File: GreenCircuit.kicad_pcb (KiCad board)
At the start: 2 copper layers, 114.9 x 97.8 mm, 71 parts, among them J1 AVR ISP 6, J2 USB_A-Connector, SW1 SW_Push, SW10 SW_Push, SW11 SW_Push, SW12 SW_Push, SW13 SW_Push, SW14 SW_Push, SW15 SW_Push, SW16 SW_Push, SW17 SW_Push, SW18 SW_Push, SW19 SW_Push, SW2 SW_Push, SW20 SW_Push, SW21 PG1350, SW22 PG1350, SW23 PG1350, SW3 SW_Push, SW4 SW_Push, SW5 SW_Push, SW6 SW_Push, SW7 SW_Push, SW8 SW_Push, SW9 SW_Push, U1 ATmega328P-PU, Y1 16MHz

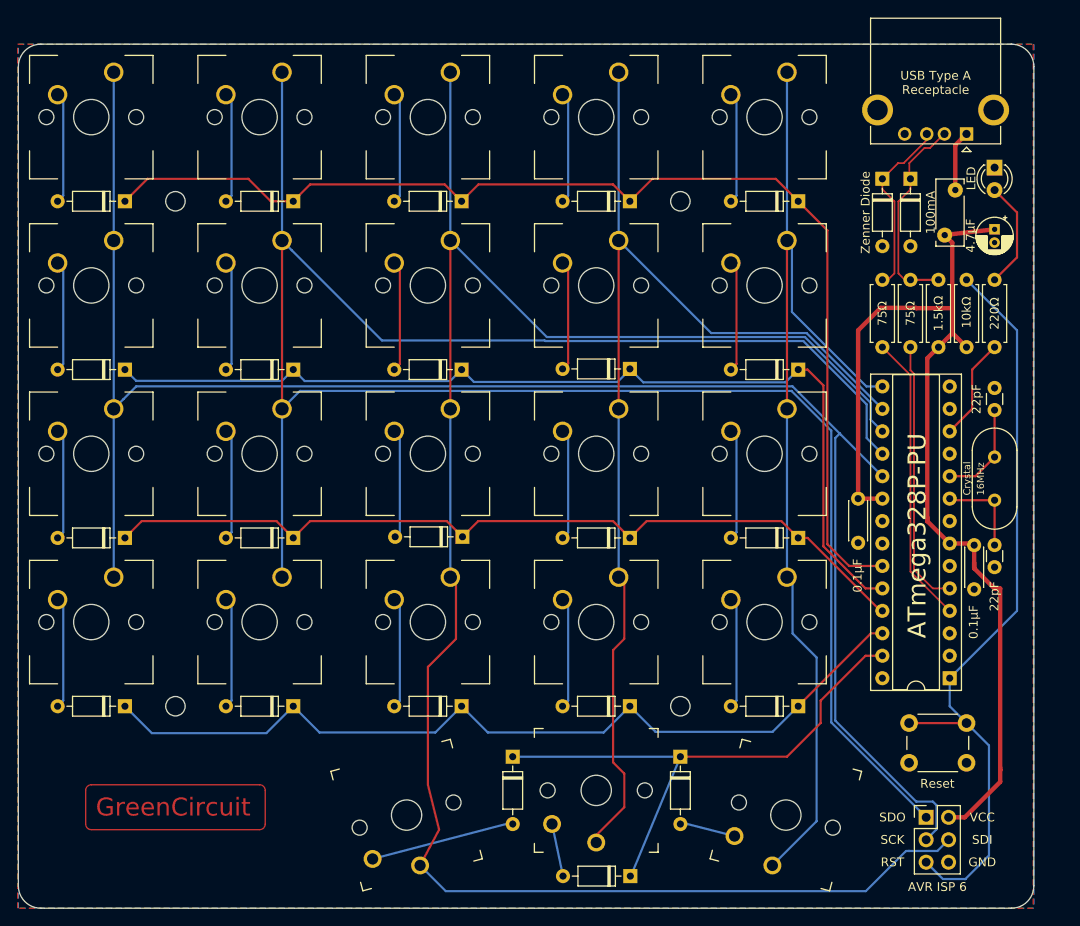
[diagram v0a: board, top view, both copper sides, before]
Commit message: v0.5
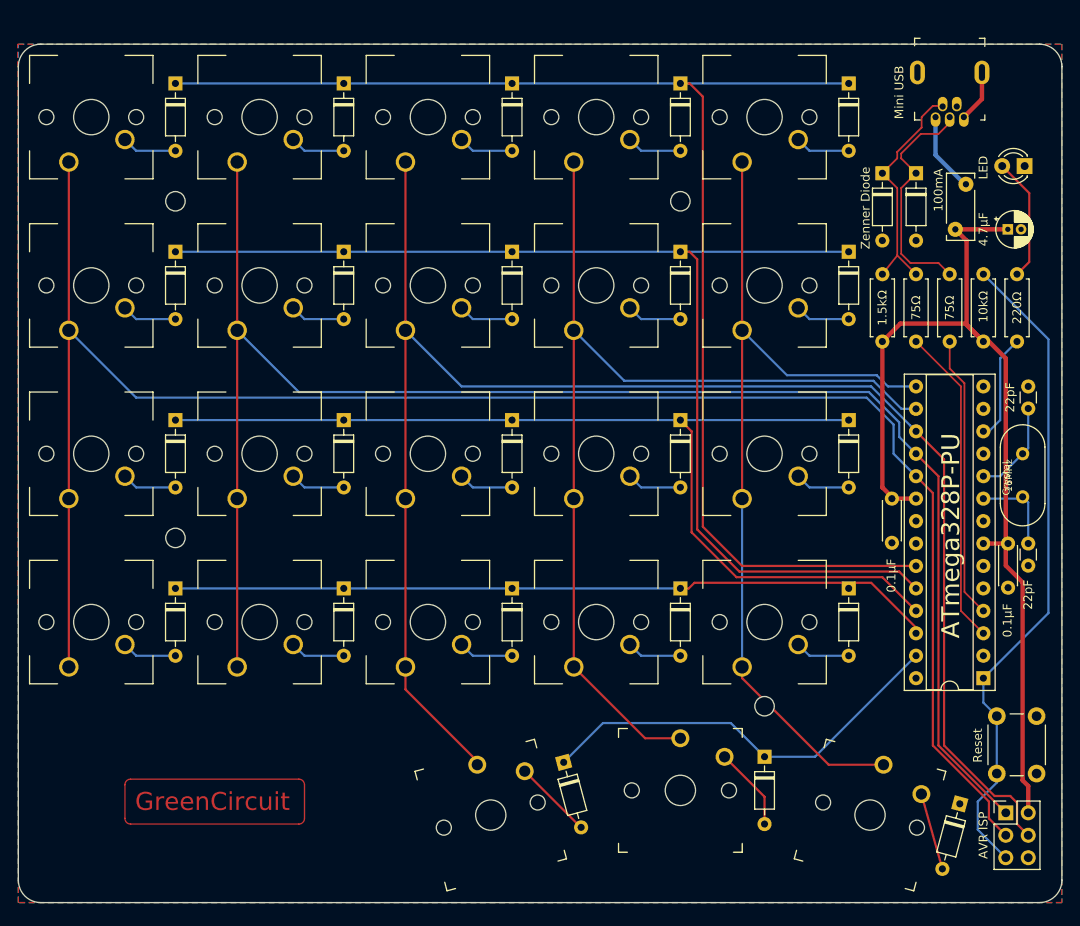
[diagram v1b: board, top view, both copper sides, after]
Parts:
- removed the J2 at (184.4, 68.4)
- removed Logo_KiCad: KiCad-Logo_20mm_SilkScreen, Symbol:KiCad-Logo_20mm_SilkScreen
- removed OSHW_Logo: OSHW-Logo2_36.5x30mm_SilkScreen, Symbol:OSHW-Logo2_36.5x30mm_SilkScreen
- added Mini USB: USB_B_Mini, digikey-footprints:USB_Mini_B_Female_548190519, F.Cu at (182.5, 66.5)
- J2: renamed from J1; value AVR ISP 6 -> AVR ISP
- moved D23 32.1 mm to (183.6, 144.2), turned to 255 degrees
- moved D22 20.3 mm to (161.5, 138.9), turned to 270 degrees
- moved H3 19.1 mm to (94.8, 114.1)
- moved D18 14.5 mm to (132.9, 119.8), turned to 270 degrees
- moved D3 14.5 mm to (132.9, 62.7), turned to 270 degrees
- moved D8 14.5 mm to (132.9, 81.7), turned to 270 degrees
- moved D1 14.5 mm to (94.8, 62.7), turned to 270 degrees
- moved D10 14.5 mm to (171.0, 81.7), turned to 270 degrees
- moved D16 14.5 mm to (94.8, 119.8), turned to 270 degrees
- moved D17 14.5 mm to (113.9, 119.8), turned to 270 degrees
- moved D19 14.5 mm to (152.0, 119.8), turned to 270 degrees
- moved D2 14.5 mm to (113.9, 62.7), turned to 270 degrees
- moved D20 14.5 mm to (171.0, 119.8), turned to 270 degrees
- moved D4 14.5 mm to (152.0, 62.7), turned to 270 degrees
- moved D5 14.5 mm to (171.0, 62.7), turned to 270 degrees
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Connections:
- U1 pad 3: (no net) -> D-
- U1 pad 5: D- -> (no net)
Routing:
- net Col1: track 251.0 -> 185.6 mm
- net Col2: track 214.6 -> 186.1 mm
- net Row1: track 111.2 -> 136.6 mm
- net Row2: track 95.4 -> 118.5 mm
- net Row0: track 131.0 -> 154.0 mm
- net Row4: track 62.7 -> 48.0 mm
- net Col4: track 115.5 -> 100.8 mm
- net Reset: track 88.1 -> 75.0 mm
- net Col3: track 127.5 -> 115.0 mm
- net Row3: track 99.0 -> 87.3 mm
- net Net-(D21-Pad2): track 16.4 -> 9.01 mm
- net +5V: track 119.1 -> 112.4 mm
- net Net-(D19-Pad2): track 12.6 -> 6.24 mm
- net Net-(D4-Pad2): track 12.6 -> 6.24 mm
- net Net-(D14-Pad2): track 12.6 -> 6.24 mm
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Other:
- board size 114.9 x 97.8 mm -> 118.1 x 97.2 mm
- board text added: "Rev 0.5 Oct 2020 James Sa"
- board text removed: "Design with"
- board text removed: "Rev 0.4 Oct 2020 James Sa"
- board text removed: "USB Type A Receptacle"
